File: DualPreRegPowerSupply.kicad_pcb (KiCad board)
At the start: 4 copper layers, 100 x 100 mm, 178 parts, among them J101 Banana_Red, J102 Banana_Black, J201 Banana_Red, J202 Banana_Black, J401 Conn_02x05_Odd_Even, J601 Power Input, J801 Conn_01x03_Pin, J802 Conn_02x02_Odd_Even, J901 Power Input, M401 Fan_4pin, Q301 MMBT3904, Q302 TIP42C, Q303 BSS138, Q401 BSS138, Q501 MMBT3906, Q801 BSS138, Q802 BSS138, U1001 AP64060QWU, U1002 AP7383, U1003 LM2776, U1005 XC6901D121MR-G, U301 TLV4387PWR, U302 LMV331, U501 LT8612, U701 ADS1118IDGS, U702 MCP48FVB22, U801 ISO6721RFBD, U802 ATtiny1614-SS, U901 AP63200WU

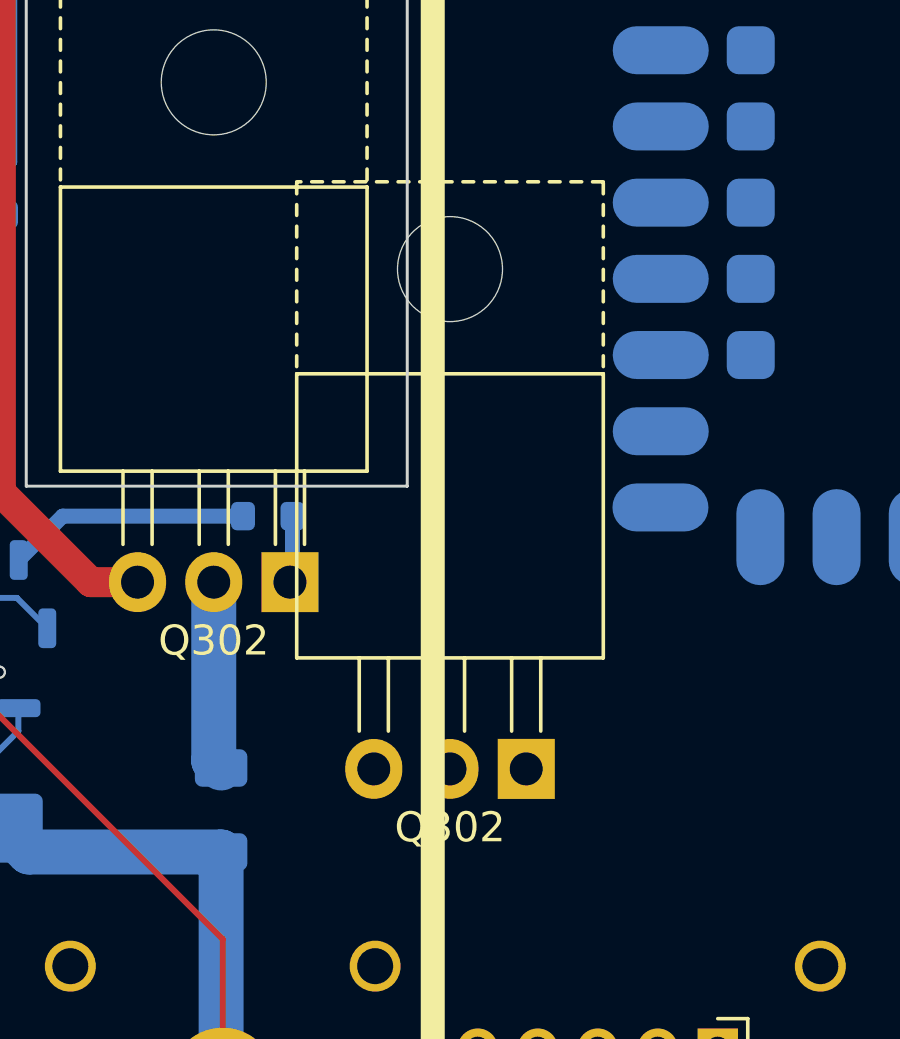
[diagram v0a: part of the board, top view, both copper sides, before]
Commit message: test commit
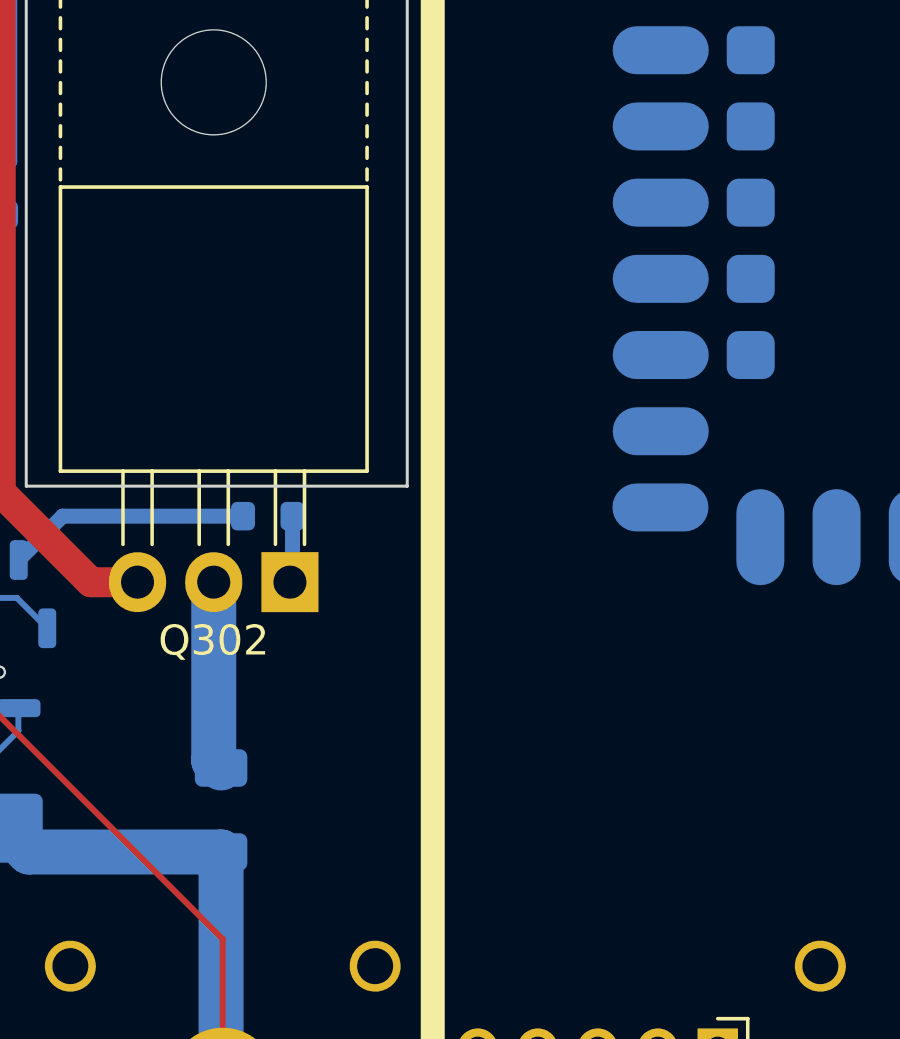
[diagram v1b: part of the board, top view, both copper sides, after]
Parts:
- removed the Q302 at (137.1, 126.6)
